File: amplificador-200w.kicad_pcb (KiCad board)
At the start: 2 copper layers, 92.5 x 81 mm, 34 parts, among them J1 IN, J10 MH, J11 MH, J12 FAN, J3 PWR, J4 out, J5 out, J6 out, J7 out, J8 MH, J9 MH, U1 TDA7850

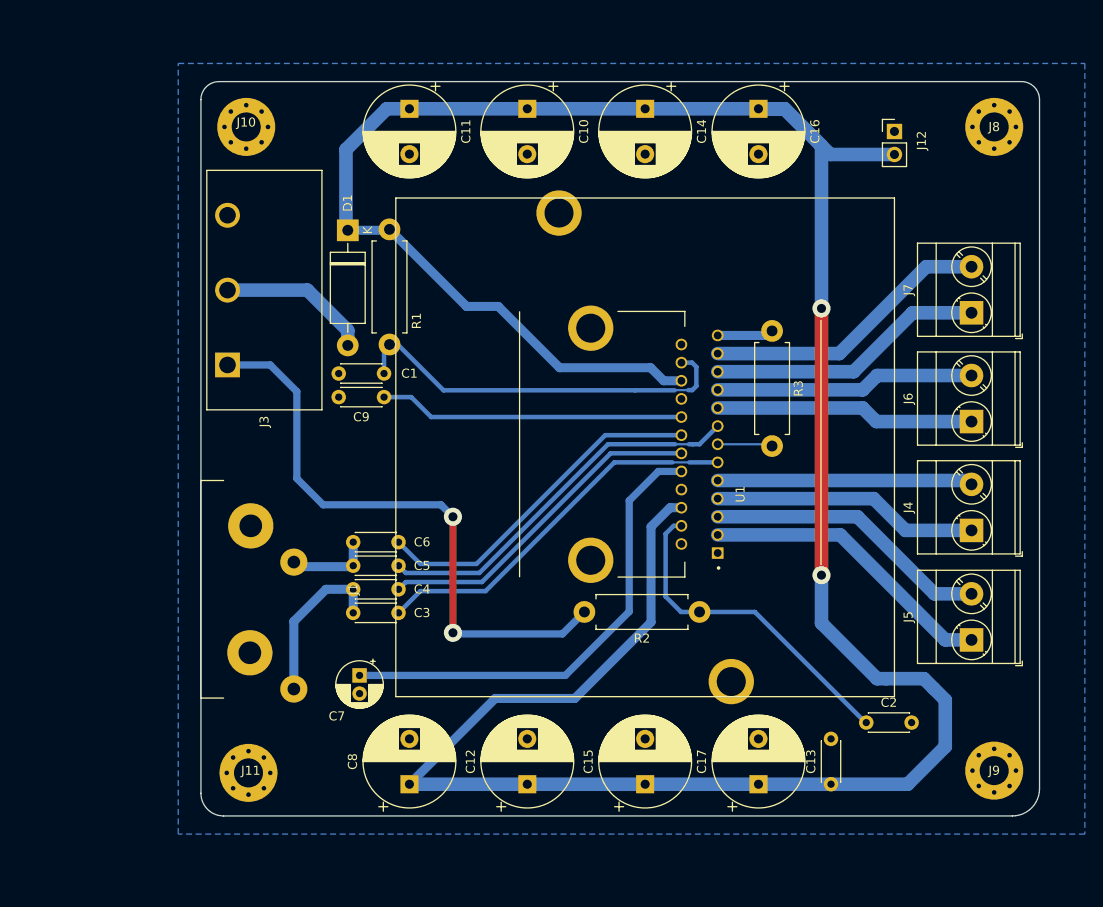
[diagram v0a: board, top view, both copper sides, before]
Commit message: version 2 enviada a fabricar
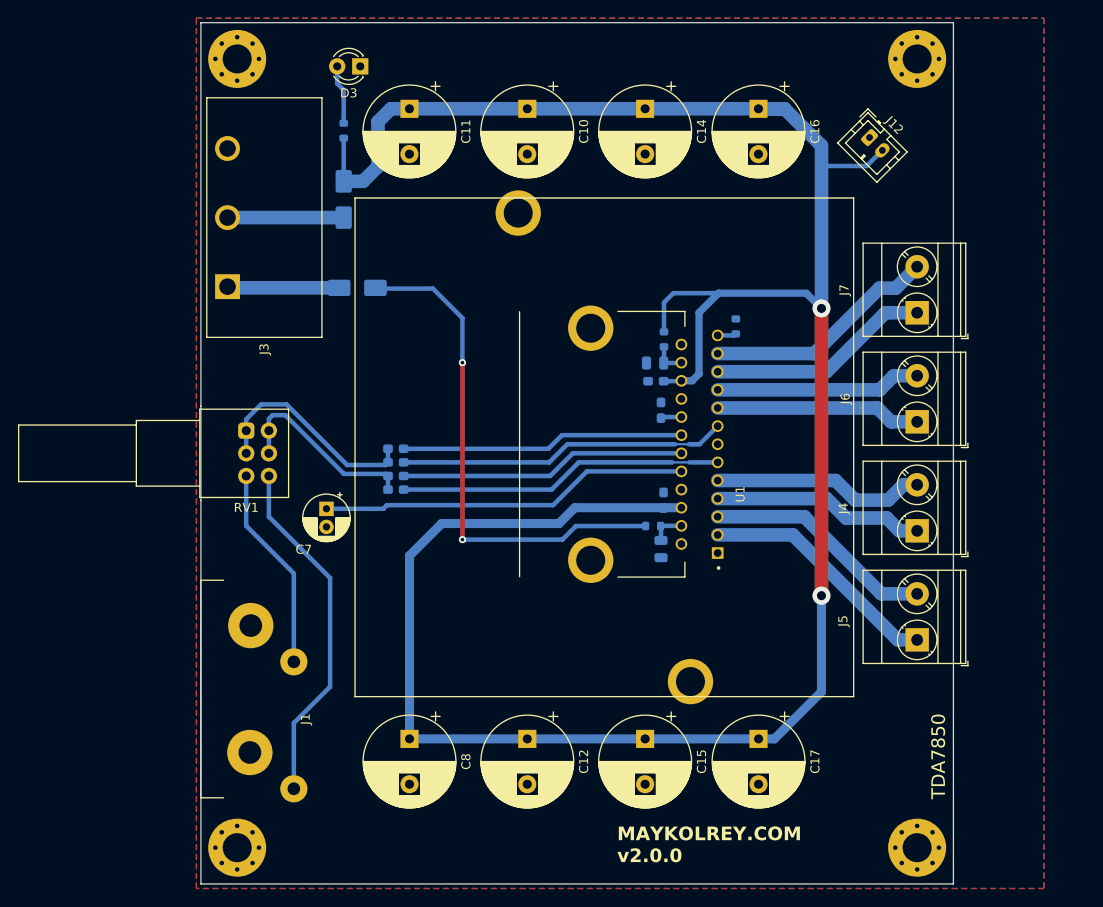
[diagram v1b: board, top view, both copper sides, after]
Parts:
- added C18: 100nF, Capacitor_SMD:C_0603_1608Metric_Pad1.08x0.95mm_HandSolder, B.Cu at (150.2, 90.0)
- added D2: D_ALT, Diode_SMD:D_SMA, B.Cu at (117.2, 79.8)
- added D3: LED, LED_THT:LED_D3.0mm, F.Cu at (117.6, 55.3)
- added G***: LOGO, MR-footprint:logo_mr_6x6mm, F.Cu at (142.4, 141.2)
- added R4: 10K, Resistor_SMD:R_0603_1608Metric, B.Cu at (115.8, 62.4)
- added RV1: R_Potentiometer_Dual, Potentiometer_THT:Potentiometer_Alps_RK097_Dual_Horizontal, F.Cu at (105.0, 95.5)
- C1, C2: footprint Capacitor_THT:C_Disc_D4.3mm_W1.9mm_P5.00mm -> Capacitor_SMD:C_0805_2012Metric; moved to B.Cu
- C13, C3, C4, C5, C6: value 0.1uF -> 100nF; footprint Capacitor_THT:C_Disc_D4.3mm_W1.9mm_P5.00mm -> Capacitor_SMD:C_0603_1608Metric_Pad1.08x0.95mm_HandSolder; moved to B.Cu
- C9: footprint Capacitor_THT:C_Disc_D4.3mm_W1.9mm_P5.00mm -> Capacitor_SMD:C_0603_1608Metric_Pad1.08x0.95mm_HandSolder; moved to B.Cu
- D1: footprint Diode_THT:D_DO-15_P12.70mm_Horizontal -> Diode_SMD:D_SMA; moved to B.Cu
- J12: footprint Connector_PinHeader_2.54mm:PinHeader_1x02_P2.54mm_Vertical -> Connector_JST:JST_PH_B2B-PH-K_1x02_P2.00mm_Vertical
- R1, R2, R3: footprint Resistor_THT:R_Axial_DIN0411_L9.9mm_D3.6mm_P12.70mm_Horizontal -> Resistor_SMD:R_0603_1608Metric; moved to B.Cu
- moved C13 36.4 mm to (151.0, 103.2)
- moved C9 30.6 mm to (150.8, 93.2), turned to 90 degrees
- moved R1 30.3 mm to (151.1, 85.4)
- moved C1 29.9 mm to (150.1, 88.0)
- moved C2 29.6 mm to (150.8, 108.6), turned to -90 degrees
- moved C7 18.7 mm to (113.8, 104.1)
- moved C3 13.6 mm to (121.5, 102.0)
- moved C4 12.5 mm to (121.5, 100.5)
- moved J9 12.0 mm to (179.0, 141.5)
- moved C5 11.4 mm to (121.5, 99.0)
- moved J8 11.3 mm to (179.0, 54.5)
- moved J1 11.0 mm to (105.5, 124.0)
- moved R2 10.8 mm to (149.9, 106.0)
- moved C6 10.3 mm to (121.5, 97.5)
- moved J11 8.34 mm to (104.0, 141.5)
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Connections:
- net VCC renamed +12V
- C3 pad 2: Net-(J1-Pin_4) -> /IN_LEFT_P
- C4 pad 2: Net-(J1-Pin_4) -> /IN_LEFT_P
- C5 pad 2: Net-(J1-Pin_2) -> /IN_RIGTH_P
- C6 pad 2: Net-(J1-Pin_2) -> /IN_RIGTH_P
- J1 pad 2: Net-(J1-Pin_2) -> /IN_RIGTH
- J1 pad 4: Net-(J1-Pin_4) -> /IN_LEFT
- J3 pad 1: /REMOTE -> Net-(D2-A)
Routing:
- net Net-(U1-MUTE): track 47.9 -> 3.76 mm
- net /IN_LEFT: track 0.00 -> 39.0 mm
- net +12V: track 310.4 -> 273.7 mm
- net Net-(U1-ST-BY): track 37.1 -> 3.91 mm
- net Net-(U1-AC-GND): track 33.7 -> 2.30 mm
- net /IN_RIGTH_P: track 0.00 -> 24.5 mm
- net /IN_RIGTH: track 0.00 -> 22.7 mm
- net /IN_LEFT_P: track 0.00 -> 21.4 mm
- net Net-(J1-Pin_4): track 18.1 -> 0.00 mm
- net Net-(D2-A): track 0.00 -> 12.4 mm
- net Net-(U1-SVR): track 52.0 -> 40.9 mm
- net /REMOTE: track 65.8 -> 56.2 mm
- net Net-(J1-Pin_2): track 9.40 -> 0.00 mm
- net Net-(U1-IN4): track 38.1 -> 31.3 mm
- net GND: track 6.64 -> 0.00 mm
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- added copper zone on F.Cu, net GND
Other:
- board size 92.5 x 81 mm -> 83 x 95 mm
- board text added: "MAYKOLREY.COM ${REVISION}"
- board text removed: "MAYKOLREY.COM"
